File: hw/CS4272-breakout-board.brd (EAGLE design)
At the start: 30.5 x 33 mm, 20 parts, among them Q1 24.576M, U1 CODEC

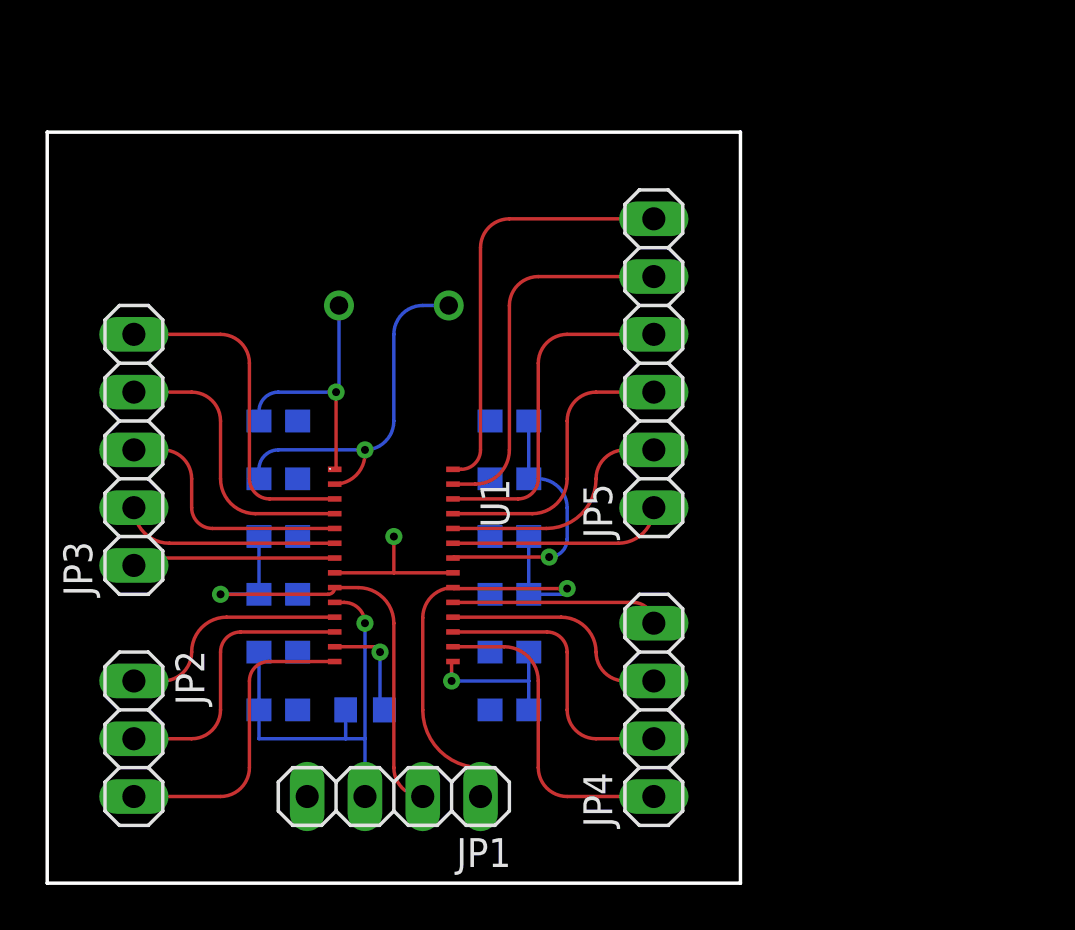
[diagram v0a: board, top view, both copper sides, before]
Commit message: Update PCB
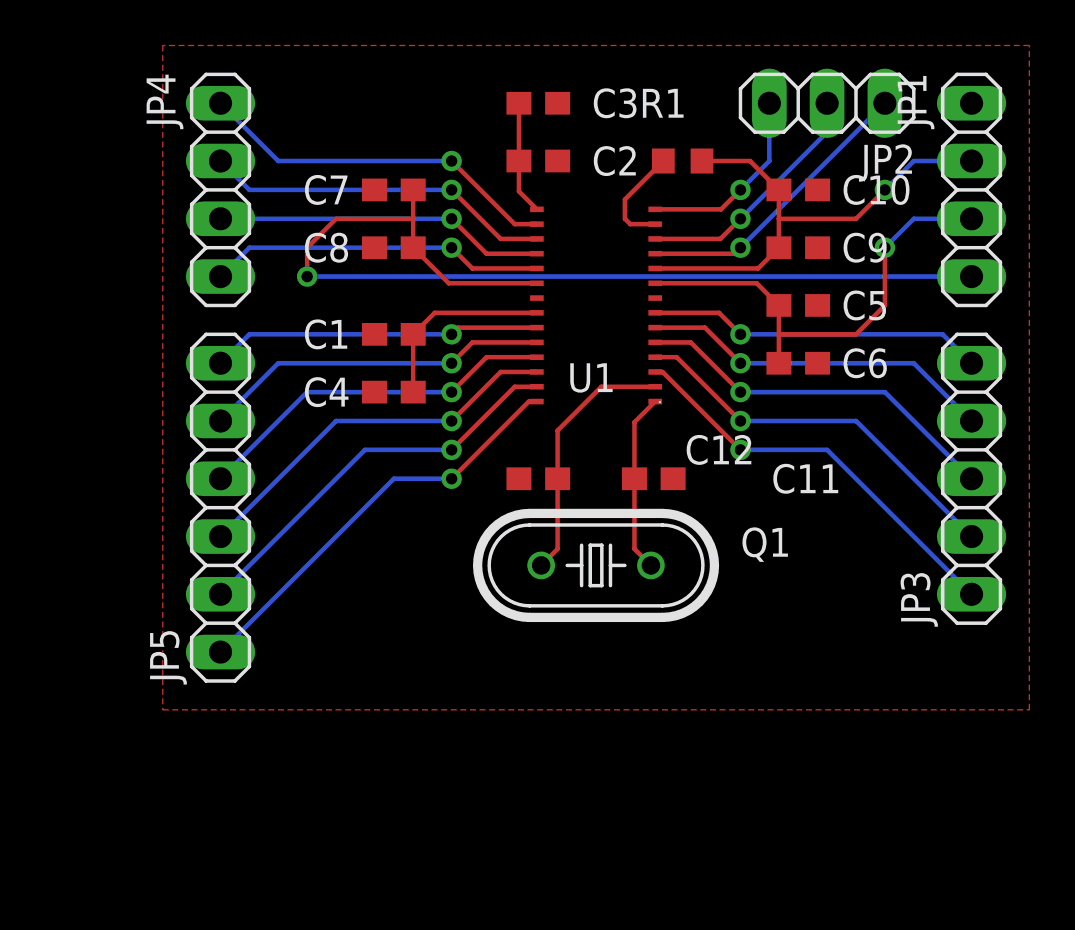
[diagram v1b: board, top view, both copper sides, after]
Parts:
- moved JP2 41.3 mm to (34.3, 34.3), turned to 180 degrees
- moved JP3 36.9 mm to (40.6, 17.8), turned to 270 degrees
- moved JP1 36.8 mm to (40.6, 30.5), turned to 90 degrees
- moved C10 30.6 mm to (33.0, 30.5), flipped to the top, turned to 0 degrees
- moved C9 30.6 mm to (33.0, 27.9), flipped to the top, turned to 0 degrees
- moved JP4 29.8 mm to (7.62, 30.5), turned to 270 degrees
- moved R1 27.9 mm to (27.9, 31.8), flipped to the top
- moved C3 26.7 mm to (21.6, 34.3), flipped to the top
- moved C5 26.2 mm to (33.0, 25.4), flipped to the top, turned to 180 degrees
- moved C6 24.1 mm to (33.0, 22.9), flipped to the top, turned to 180 degrees
- moved C2 21.6 mm to (21.6, 31.8), flipped to the top
- moved JP5 20.1 mm to (7.62, 16.5), turned to 270 degrees
- moved C12 16.7 mm to (26.7, 17.8), flipped to the top, turned to 180 degrees
- moved C7 16.1 mm to (15.2, 30.5), flipped to the top, turned to 180 degrees
- moved C8 16.1 mm to (15.2, 27.9), flipped to the top, turned to 180 degrees
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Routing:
- net VA: track 20.2 -> 44.3 mm
- net GND: track 6.79 -> 0.00 mm, vias 1 -> 0
- net SDOUT: track 9.48 -> 15.6 mm, vias 0 -> 1
- net SDIN: track 8.96 -> 14.8 mm, vias 0 -> 1
- net AINB-: track 9.21 -> 14.8 mm, vias 0 -> 1
- net SCLK: track 11.0 -> 16.4 mm, vias 0 -> 1
- net !RST!: track 13.5 -> 8.44 mm, vias 0 -> 1
- net !AMUTEC!: track 9.48 -> 14.6 mm, vias 0 -> 1
- net AOUTA-: track 10.3 -> 15.3 mm, vias 0 -> 1
- net N$2: track 16.0 -> 11.3 mm, vias 1 -> 0
- net LRCK: track 12.5 -> 17.2 mm, vias 0 -> 1
- net AINB+: track 9.99 -> 14.5 mm, vias 0 -> 1
- net AOUTA+: track 12.5 -> 16.1 mm, vias 0 -> 1
- net N$1: track 11.4 -> 7.88 mm, vias 1 -> 0
- net MCLK: track 14.8 -> 18.0 mm, vias 0 -> 1
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- added copper zone on layer 1, net GND
- removed copper zone on layer 16, net GND
- removed copper zone on layer 1, net N$3
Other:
- board outline removed
